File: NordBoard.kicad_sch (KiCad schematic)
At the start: 99 parts, among them P1 USB_C_Plug_USB2.0, P2 USB_C_Plug_USB2.0, SW1 SW_Push, SW10 SW_Push, SW11 SW_Push, SW12 SW_Push, SW13 SW_Push, SW14 SW_Push, SW15 SW_Push, SW16 SW_Push, SW17 SW_Push, SW18 SW_Push, SW19 SW_Push, SW2 SW_Push, SW20 SW_Push, SW21 SW_Push, SW22 SW_Push, SW23 SW_Push, SW24 SW_Push, SW25 SW_Push, SW26 SW_Push, SW27 SW_Push, SW28 SW_Push, SW29 SW_Push, SW3 SW_Push, SW30 SW_Push, SW31 SW_Push, SW32 SW_Push, SW33 SW_Push, SW34 SW_Push, SW35 SW_Push, SW36 SW_Push, SW37 SW_Push, SW38 SW_Push, SW39 SW_Push, SW4 SW_Push, SW40 SW_Push, SW5 SW_Push, SW50 SW_Push, SW51 SW_Push, SW6 SW_Push, SW7 SW_Push, SW8 SW_Push, SW9 SW_Push, U1 XIAO-RP2040-DIP, U2 XIAO-RP2040-DIP

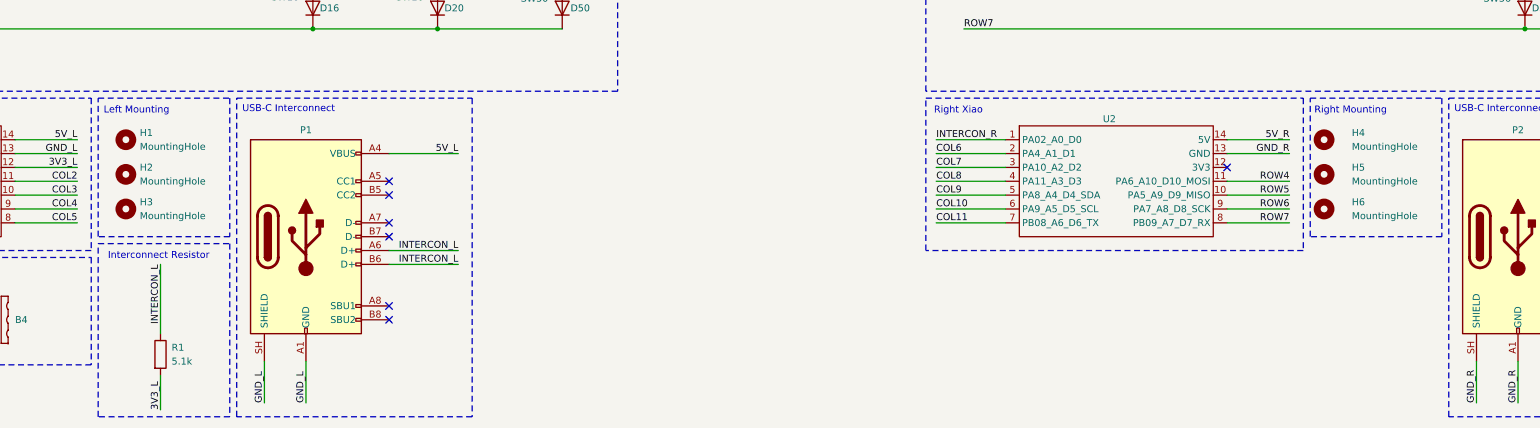
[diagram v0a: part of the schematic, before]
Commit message: feat: gerbers, new journal, update readme, finish BOM
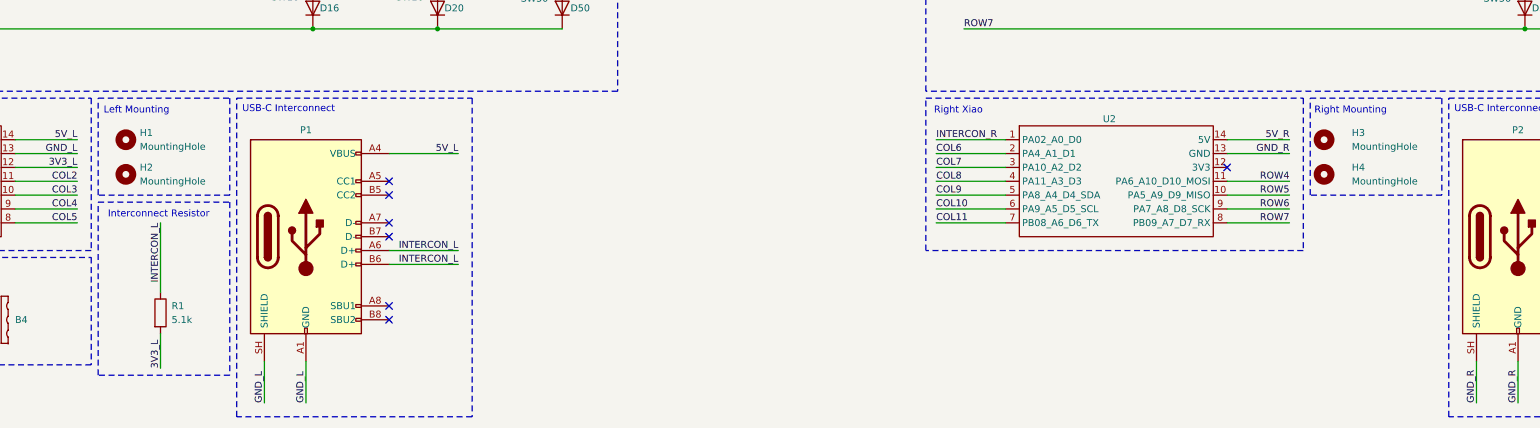
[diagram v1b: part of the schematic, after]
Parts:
- removed H3, H6: MountingHole, MountingHole:MountingHole_2.2mm_M2, symbol Mechanical:MountingHole
- renumbered H4 to H3, H5 to H4
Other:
- moved on the sheet: R1
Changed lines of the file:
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@@
 	(rectangle
 		(start 86.36 106.68)
-		(end 110.49 132.08)
+		(end 110.49 124.46)
 		(stroke
 			(width 0)
@@
 	)
 	(rectangle
-		(start 86.36 133.35)
-		(end 110.49 165.1)
+		(start 86.36 125.73)
+		(end 110.49 157.48)
 		(stroke
 			(width 0)
@@
 	(rectangle
 		(start 308.61 106.68)
-		(end 332.74 132.08)
+		(end 332.74 124.46)
 		(stroke
 			(width 0)
@@
 	(text "Interconnect Resistor"
 		(exclude_from_sim no)
-		(at 88.138 135.636 0)
+		(at 88.138 128.016 0)
 		(effects
 			(font
@@
 	(wire
 		(pts
-			(xy 97.79 137.16) (xy 97.79 149.86)
+			(xy 97.79 129.54) (xy 97.79 142.24)
 		)
 		(stroke
@@
 	(wire
 		(pts
-			(xy 97.79 157.48) (xy 97.79 163.83)
+			(xy 97.79 149.86) (xy 97.79 156.21)
 		)
 		(stroke
@@
 	)
 	(label "3V3_L"
-		(at 97.79 163.83 90)
+		(at 97.79 156.21 90)
 		(effects
 			(font
@@
 	)
 	(label "INTERCON_L"
-		(at 97.79 137.16 270)
+		(at 97.79 129.54 270)
 		(effects
 			(font
@@
 		(in_pos_files yes)
 		(dnp no)
-		(property "Reference" "H4"
+		(property "Reference" "H3"
 			(at 316.23 113.0299 0)
 			(show_name no)
@@
 			(project "NordBoard"
 				(path "/7cf7f72d-7ab1-4807-b592-339093d5ca44"
-					(reference "H4")
+					(reference "H3")
 					(unit 1)
 				)
@@
 	)
 	(symbol
-		(lib_id "Mechanical:MountingHole")
-		(at 91.44 127 0)
-		(unit 1)
-		(body_style 1)
-		(exclude_from_sim no)
-		(in_bom no)
-		(on_board yes)
-		(in_pos_files yes)
-		(dnp no)
-		(fields_autoplaced yes)
-		(property "Reference" "H3"
-			(at 93.98 125.7299 0)
-			(show_name no)
-			(do_not_autoplace no)
-			(effects
-				(font
-					(size 1.27 1.27)
-				)
-				(justify left)
-			)
-		)
-		(property "Value" "MountingHole"
-			(at 93.98 128.2699 0)
-			(show_name no)
-			(do_not_autoplace no)
-			(effects
-				(font
-					(size 1.27 1.27)
-				)
-				(justify left)
-			)
-		)
-		(property "Footprint" "MountingHole:MountingHole_2.2mm_M2"
-			(at 91.44 127 0)
-			(hide yes)
-			(show_name no)
-			(do_not_autoplace no)
-			(effects
-				(font
-					(size 1.27 1.27)
-				)
-			)
-		)
-		(property "Datasheet" ""
-			(at 91.44 127 0)
-			(hide yes)
-			(show_name no)
-			(do_not_autoplace no)
-			(effects
-				(font
-					(size 1.27 1.27)
-				)
-			)
-		)
-		(property "Description" "Mounting Hole without connection"
-			(at 91.44 127 0)
-			(hide yes)
-			(show_name no)
-			(do_not_autoplace no)
-			(effects
-				(font
-					(size 1.27 1.27)
-				)
-			)
-		)
-		(instances
-			(project "NordBoard"
-				(path "/7cf7f72d-7ab1-4807-b592-339093d5ca44"
-					(reference "H3")
-					(unit 1)
-				)
-			)
-		)
-	)
-	(symbol
 		(lib_id "Device:D")
 		(at 102.87 41.91 90)
@@
 		(in_pos_files yes)
 		(dnp no)
-		(property "Reference" "H5"
+		(property "Reference" "H4"
 			(at 316.23 119.3799 0)
 			(show_name no)
@@
 			(project "NordBoard"
 				(path "/7cf7f72d-7ab1-4807-b592-339093d5ca44"
-					(reference "H5")
+					(reference "H4")
 					(unit 1)
 				)
@@
 	)
 	(symbol
-		(lib_id "Mechanical:MountingHole")
-		(at 311.15 127 0)
-		(unit 1)
-		(body_style 1)
-		(exclude_from_sim no)
-		(in_bom no)
-		(on_board yes)
-		(in_pos_files yes)
-		(dnp no)
-		(property "Reference" "H6"
-			(at 316.23 125.7299 0)
-			(show_name no)
-			(do_not_autoplace no)
-			(effects
-				(font
-					(size 1.27 1.27)
-				)
-				(justify left)
-			)
-		)
-		(property "Value" "MountingHole"
-			(at 316.23 128.2699 0)
-			(show_name no)
-			(do_not_autoplace no)
-			(effects
-				(font
-					(size 1.27 1.27)
-				)
-				(justify left)
-			)
-		)
-		(property "Footprint" "MountingHole:MountingHole_2.2mm_M2"
-			(at 311.15 127 0)
-			(hide yes)
-			(show_name no)
-			(do_not_autoplace no)
-			(effects
-				(font
-					(size 1.27 1.27)
-				)
-			)
-		)
-		(property "Datasheet" ""
-			(at 311.15 127 0)
-			(hide yes)
-			(show_name no)
-			(do_not_autoplace no)
-			(effects
-				(font
-					(size 1.27 1.27)
-				)
-			)
-		)
-		(property "Description" "Mounting Hole without connection"
-			(at 311.15 127 0)
-			(hide yes)
-			(show_name no)
-			(do_not_autoplace no)
-			(effects
-				(font
-					(size 1.27 1.27)
-				)
-			)
-		)
-		(instances
-			(project "NordBoard"
-				(path "/7cf7f72d-7ab1-4807-b592-339093d5ca44"
-					(reference "H6")
-					(unit 1)
-				)
-			)
-		)
-	)
-	(symbol
 		(lib_id "Switch:SW_Push")
 		(at 143.51 55.88 0)
@@
 	(symbol
 		(lib_id "Device:R")
-		(at 97.79 153.67 0)
+		(at 97.79 146.05 0)
 		(unit 1)
 		(body_style 1)
@@
 		(dnp no)
 		(property "Reference" "R1"
-			(at 99.822 152.4 0)
+			(at 99.822 144.78 0)
 			(show_name no)
 			(do_not_autoplace no)
@@
 		)
 		(property "Value" "5.1k"
-			(at 99.822 154.94 0)
+			(at 99.822 147.32 0)
 			(show_name no)
 			(do_not_autoplace no)
@@
 		)
 		(property "Footprint" "Resistor_SMD:R_0805_2012Metric_Pad1.20x1.40mm_HandSolder"
-			(at 96.012 153.67 90)
+			(at 96.012 146.05 90)
 			(hide yes)
 			(show_name no)
@@
 		)
 		(property "Datasheet" ""
-			(at 97.79 153.67 0)
+			(at 97.79 146.05 0)
 			(hide yes)
 			(show_name no)
@@
 		)
 		(property "Description" "Resistor"
-			(at 97.79 153.67 0)
+			(at 97.79 146.05 0)
 			(hide yes)
 			(show_name no)
